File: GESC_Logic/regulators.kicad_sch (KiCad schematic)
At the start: 46 parts, among them J1 POWER, Q1 BSC320N20NS3G, Q3 BSC320N20NS3G, U1 XL1509-5.0, U11 LM5146RGYR, U2 LM1117DT-3.3

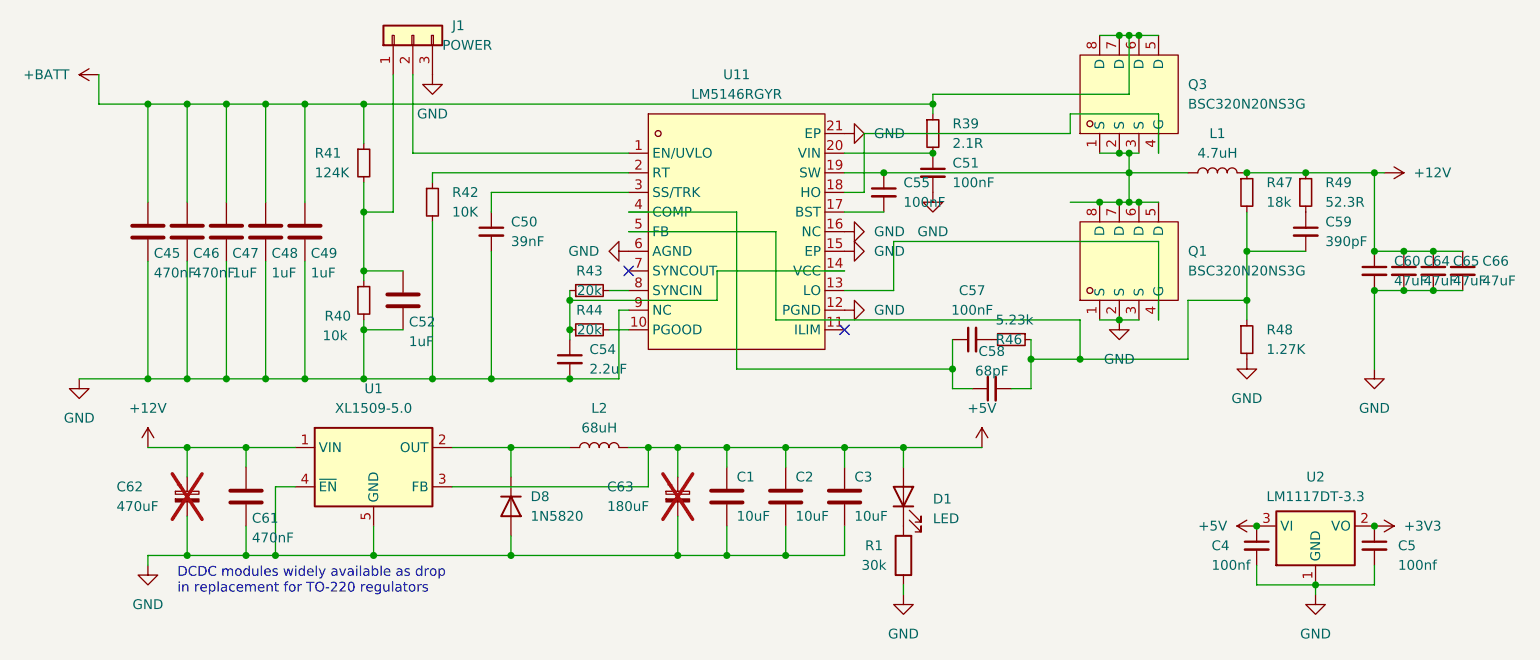
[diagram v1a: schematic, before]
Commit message: asdf
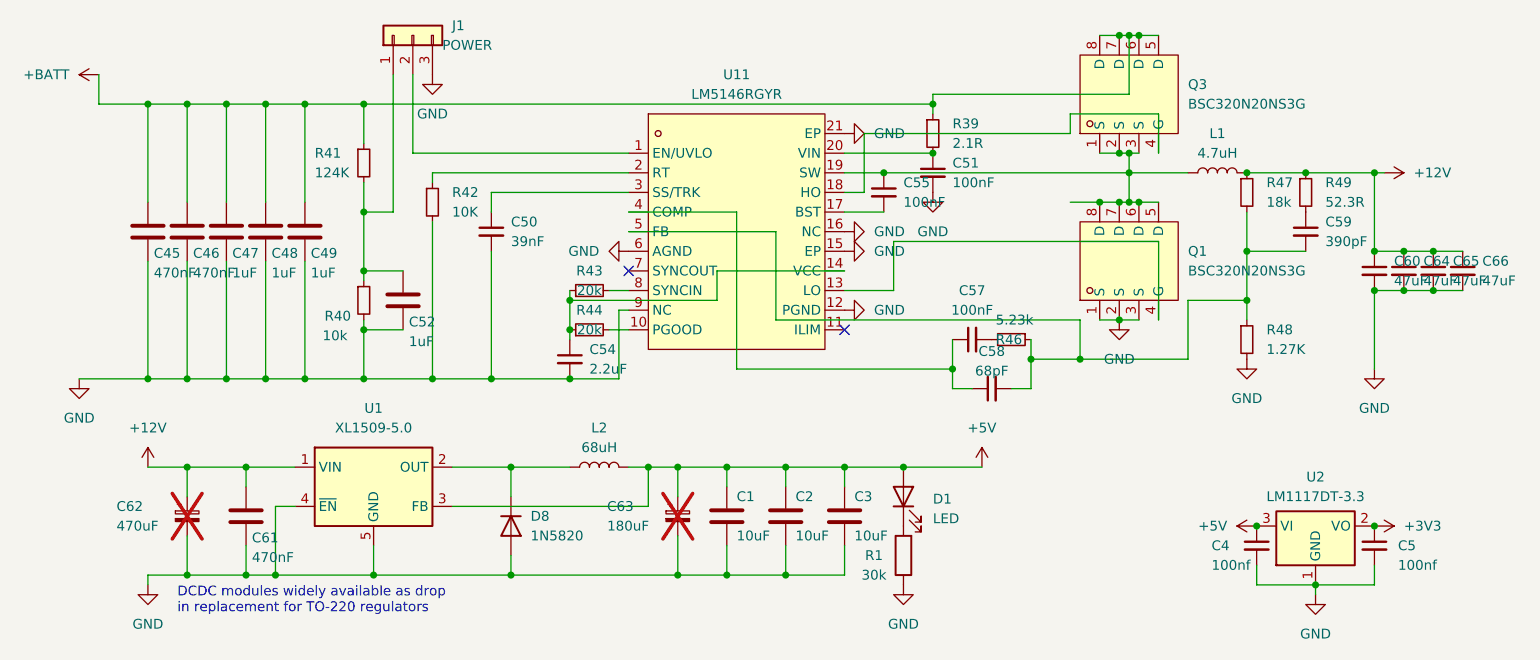
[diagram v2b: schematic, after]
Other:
- moved on the sheet: C1, C2, C3, C61, C62, C63, D8, L2, U1
